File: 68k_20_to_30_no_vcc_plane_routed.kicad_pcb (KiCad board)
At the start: 4 copper layers, 86 x 78.5 mm, 6 parts, among them U1 68030, U2 68020

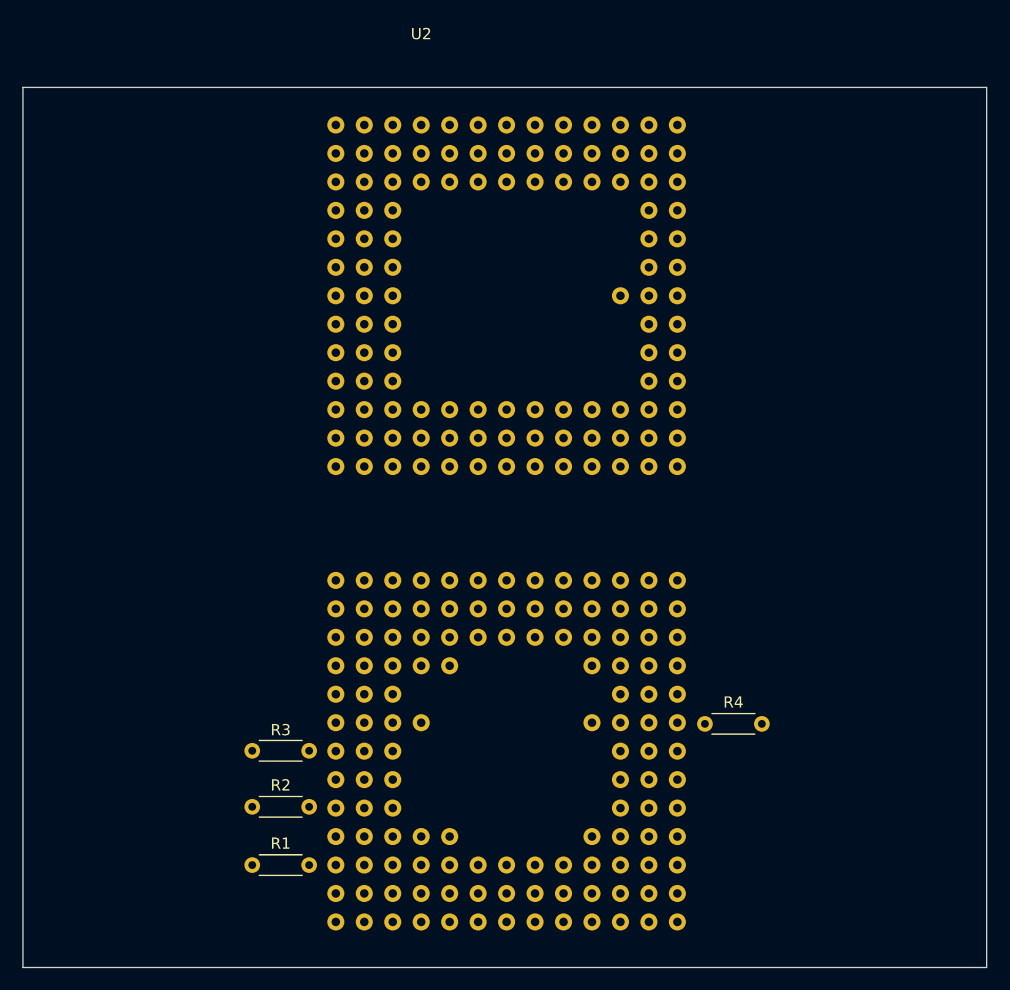
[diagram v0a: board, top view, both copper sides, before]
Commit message: Adding current state of routing.
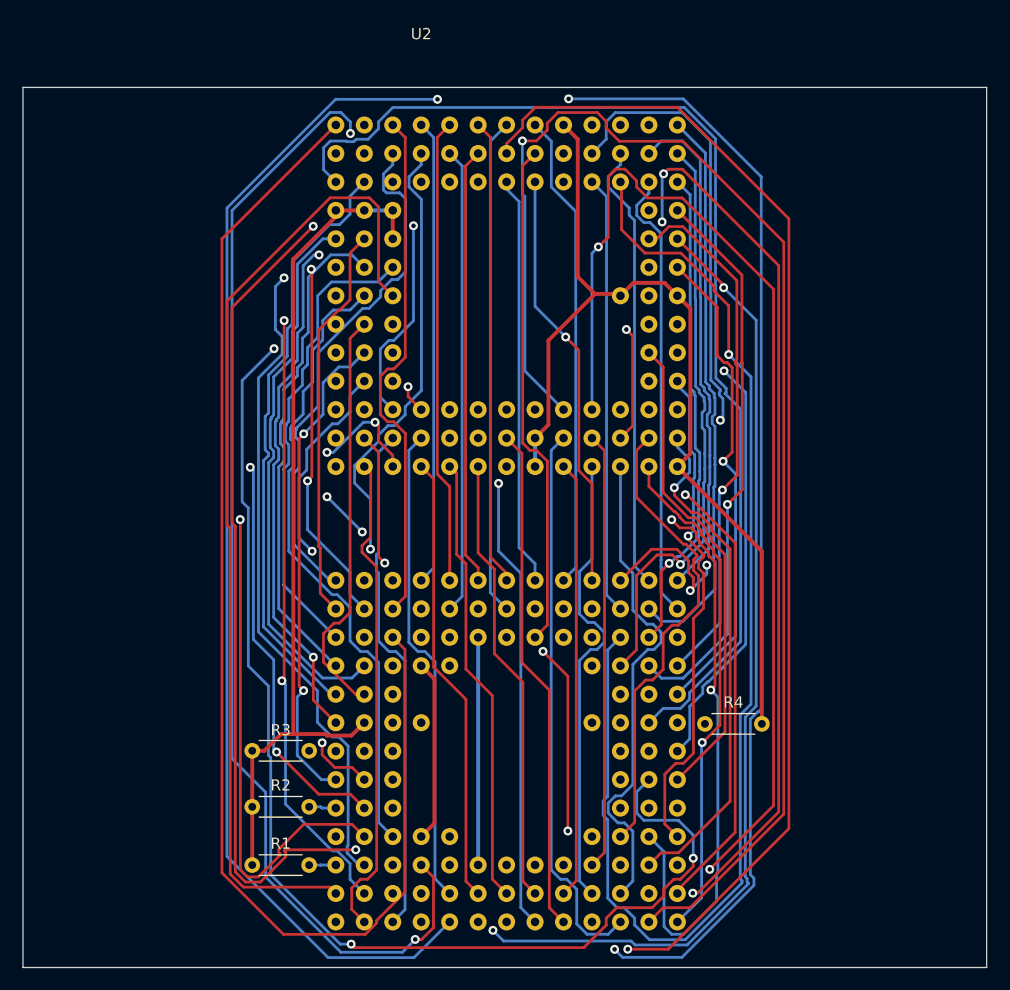
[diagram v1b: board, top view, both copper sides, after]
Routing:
- net VCC: track 0.00 -> 263.3 mm
- net /A20: track 0.00 -> 139.7 mm, vias 0 -> 3
- net /D23: track 0.00 -> 135.0 mm, vias 0 -> 1
- net /D15: track 0.00 -> 131.5 mm, vias 0 -> 2
- net /D30: track 0.00 -> 130.8 mm, vias 0 -> 3
- net /D11: track 0.00 -> 122.4 mm, vias 0 -> 1
- net /BGACK: track 0.00 -> 114.4 mm
- net /OCS: track 0.00 -> 114.3 mm, vias 0 -> 2
- net Net-(U1-CDIS): track 0.00 -> 111.8 mm, vias 0 -> 3
- net /A9: track 0.00 -> 109.8 mm, vias 0 -> 1
- net /D6: track 0.00 -> 104.4 mm, vias 0 -> 4
- net /D7: track 0.00 -> 104.0 mm, vias 0 -> 2
- net /R_W: track 0.00 -> 103.8 mm, vias 0 -> 2
- net /RESET: track 0.00 -> 99.0 mm
- net /DBEN: track 0.00 -> 87.5 mm
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- removed copper zone on In1.Cu, net VCC
